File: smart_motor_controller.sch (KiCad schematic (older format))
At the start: 44 parts, among them J10 USB_B_Micro, J101 Conn_02x04_Odd_Even, J102 I2C_CONN, J103 CAN_CONN, J104 Conn_02x05_Odd_Even, J9 Input 12V, Q101 FDD6685, SW102 SW_NRST, SW103 SW_NRST, U2 STM32F405RGT6, U3 USBLC6-2SC6

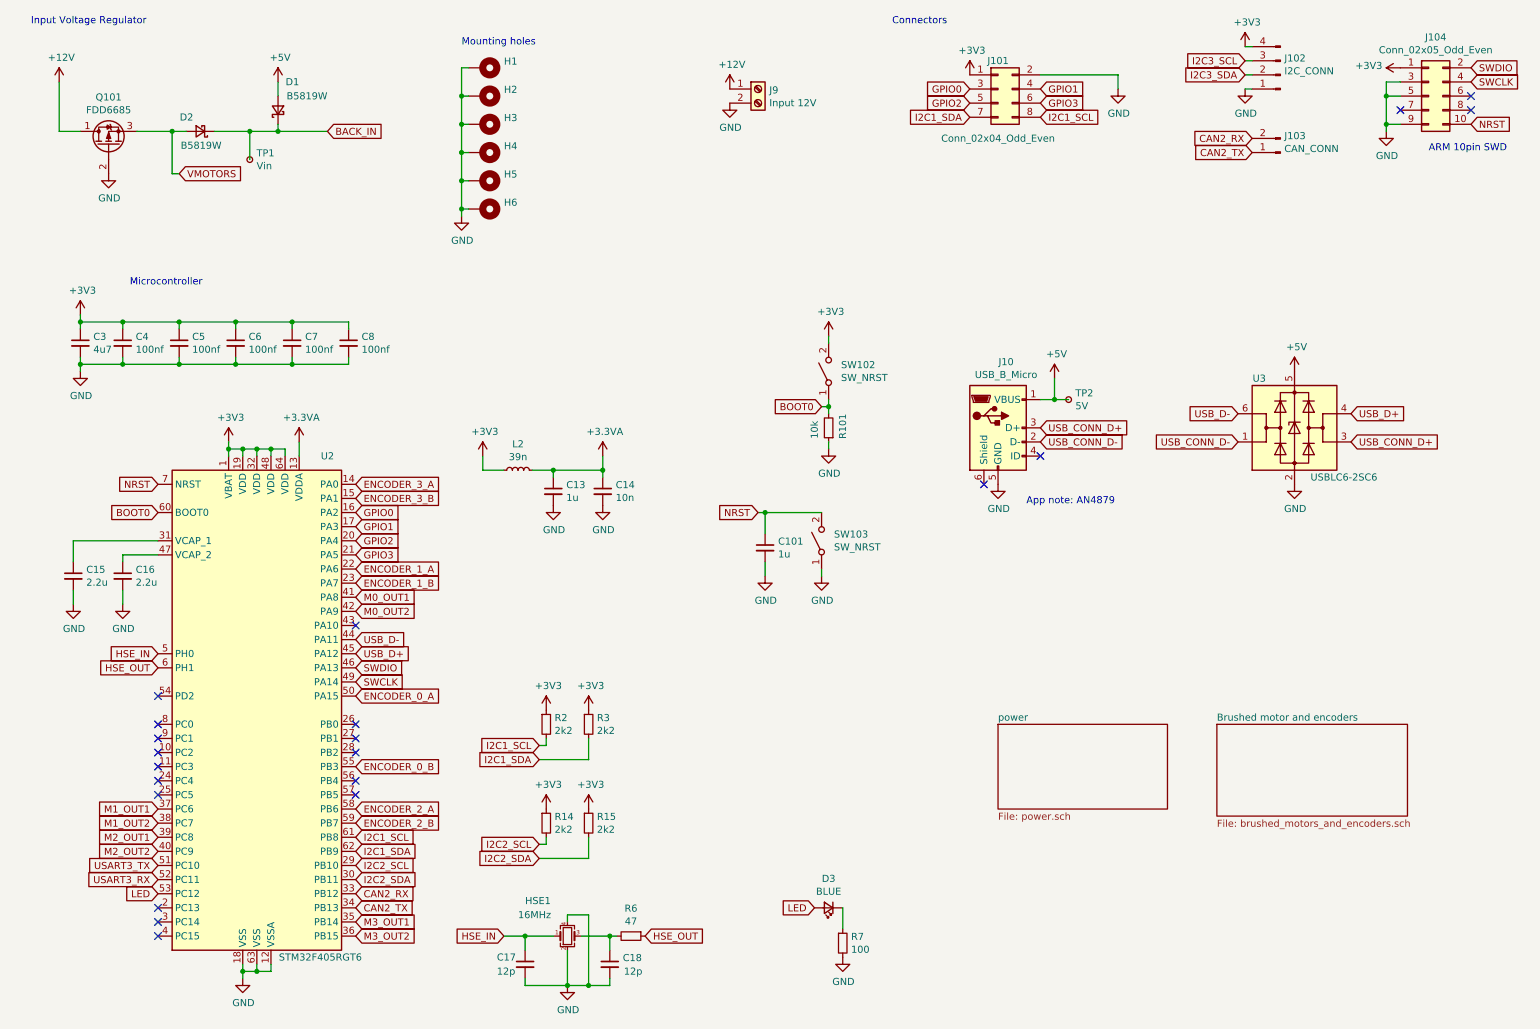
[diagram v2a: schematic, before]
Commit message: Layout
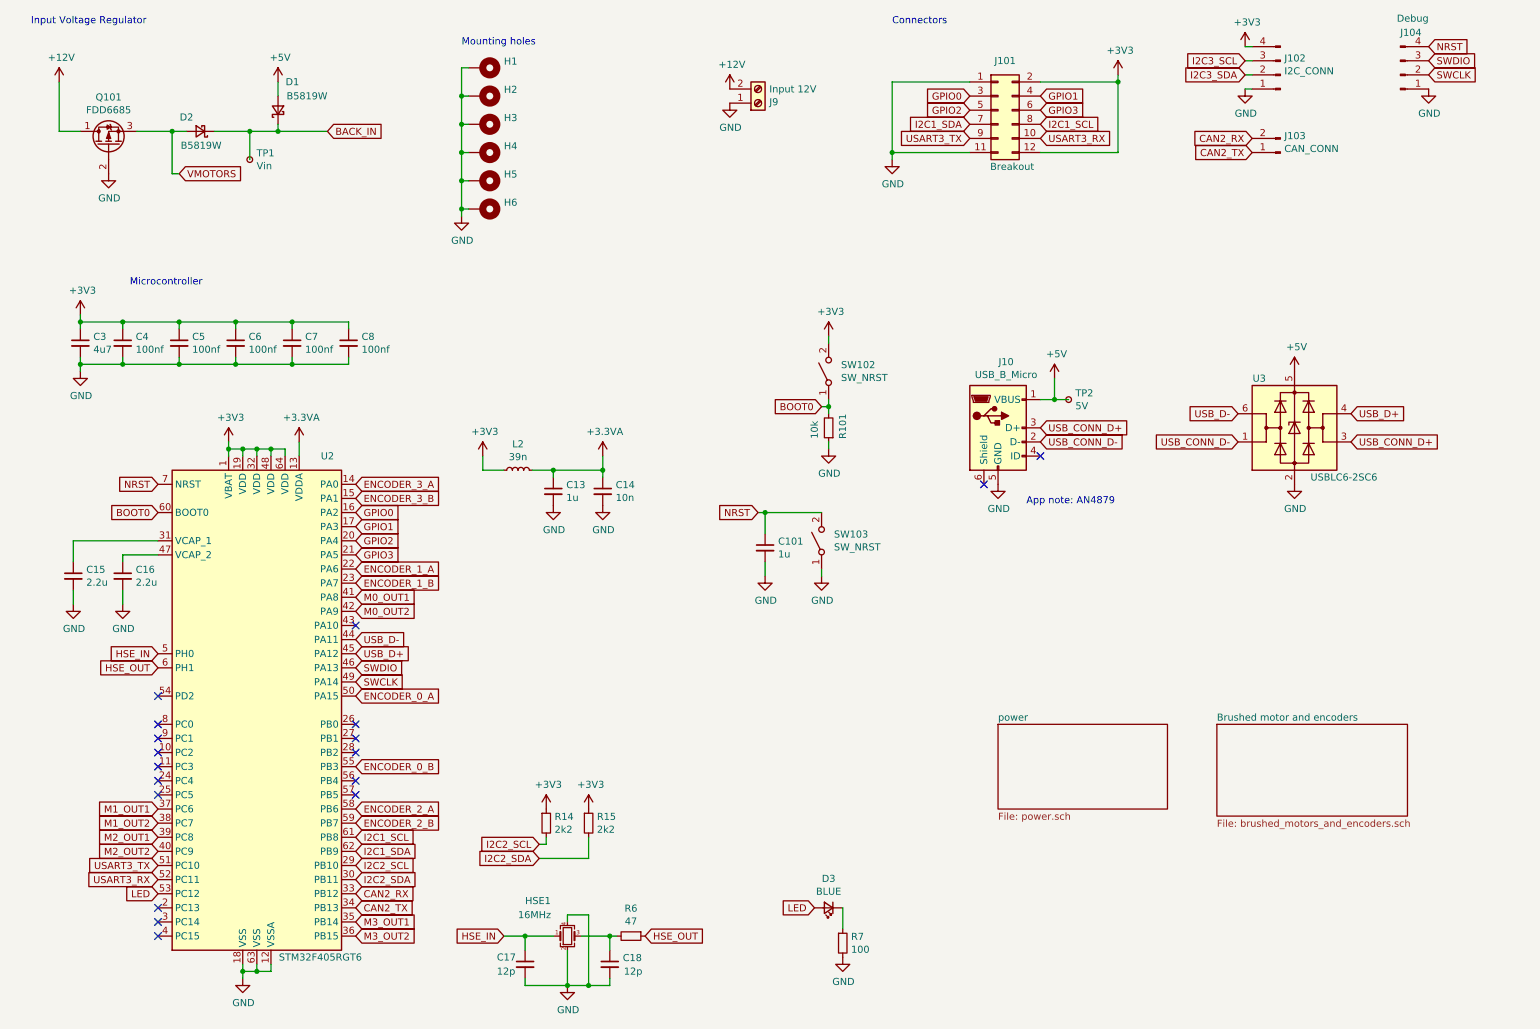
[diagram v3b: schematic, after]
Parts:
- removed J101: Conn_02x04_Odd_Even, Connector_PinHeader_2.54mm:PinHeader_2x04_P2.54mm_Vertical, symbol Connector_Generic:Conn_02x04_Odd_Even
- removed J104: Conn_02x05_Odd_Even, Connector_PinHeader_1.27mm:PinHeader_2x05_P1.27mm_Vertical_SMD, symbol Connector_Generic:Conn_02x05_Odd_Even
- removed R2, R3: 2k2, Resistor_THT:R_Axial_DIN0204_L3.6mm_D1.6mm_P5.08mm_Horizontal, symbol Device:R_Small
- added J101: Breakout, Connector_PinHeader_2.54mm:PinHeader_2x06_P2.54mm_Vertical, symbol Connector_Generic:Conn_02x06_Odd_Even
- added J104: Debug, Connector_PinHeader_2.54mm:PinHeader_1x04_P2.54mm_Vertical, symbol Connector:Conn_01x04_Male
- J9: footprint VsReality_Footprints:DB128L_5.08_2P_GN_S -> VsReality_Footprints:Ningbo_Kangnex_Elec_WJ128V_5_0_2P
- SW102, SW103: footprint (none) -> VsReality_Footprints:Diptronics MPTFP2-V-TR SMD 2.9x3.9x2mm; LCSC Part # (none) -> C495942
- TP1: footprint TestPoint:TestPoint_Pad_D2.0mm -> TestPoint:TestPoint_Pad_D1.5mm
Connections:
- net +12V: now also J9.2 (Pin_2); no longer J9.1 (Pin_1)
- net +3V3: now also J101.12 (Pin_12), J101.2 (Pin_2)
- net GND: now also J9.1 (Pin_1), J101.1 (Pin_1), J101.11 (Pin_11), J104.1 (Pin_1); no longer J9.2 (Pin_2)
- net GPIO0: now also J101.3 (Pin_3)
- net GPIO1: now also J101.4 (Pin_4)
- net GPIO2: now also J101.5 (Pin_5)
- net GPIO3: now also J101.6 (Pin_6)
- net I2C1_SCL: now also J101.8 (Pin_8)
- net I2C1_SDA: now also J101.7 (Pin_7)
- net NRST: now also J104.4 (Pin_4)
- net SWCLK: now also J104.2 (Pin_2)
- net SWDIO: now also J104.3 (Pin_3)
- net USART3_RX: now also J101.10 (Pin_10)
- net USART3_TX: now also J101.9 (Pin_9)
- no-connect marks 21 -> 18
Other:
- note removed: "ARM 10pin SWD\n"
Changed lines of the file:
@@
 Text GLabel 2900 5300 2    50   Input ~ 0
 SWCLK
-$Comp
-L Connector_Generic:Conn_02x05_Odd_Even J104
-U 1 1 6015F5C6
-P 10500 1150
-F 0 "J104" H 10550 1567 50  0000 C CNN
-F 1 "Conn_02x05_Odd_Even" H 10550 1476 50  0000 C CNN
-F 2 "Connector_PinHeader_1.27mm:PinHeader_2x05_P1.27mm_Vertical_SMD" H 10500 1150 50  0001 C CNN
-F 3 "~" H 10500 1150 50  0001 C CNN
-	1    10500 1150
-	1    0    0    -1
-$EndComp
-$Comp
-L power:GND #PWR07
-U 1 1 60160243
-P 10200 1400
-F 0 "#PWR07" H 10200 1150 50  0001 C CNN
-F 1 "GND" H 10205 1227 50  0000 C CNN
-F 2 "" H 10200 1400 50  0001 C CNN
-F 3 "" H 10200 1400 50  0001 C CNN
-	1    10200 1400
-	1    0    0    -1
-$EndComp
-Wire Wire Line
-	10300 1050 10200 1050
-Wire Wire Line
-	10200 1050 10200 1150
-Wire Wire Line
-	10300 1150 10200 1150
-Connection ~ 10200 1150
-Wire Wire Line
-	10200 1150 10200 1350
-Wire Wire Line
-	10300 1350 10200 1350
-Connection ~ 10200 1350
-Wire Wire Line
-	10200 1350 10200 1400
-$Comp
-L power:+3V3 #PWR05
-U 1 1 6016A0E3
-P 10300 950
-F 0 "#PWR05" H 10300 800 50  0001 C CNN
-F 1 "+3V3" V 10315 1078 50  0000 L CNN
-F 2 "" H 10300 950 50  0001 C CNN
-F 3 "" H 10300 950 50  0001 C CNN
-	1    10300 950
-	0    -1   -1   0
-$EndComp
-NoConn ~ 10300 1250
-NoConn ~ 10800 1250
-Text GLabel 10800 1350 2    50   Input ~ 0
-NRST
-Text GLabel 10800 1050 2    50   Input ~ 0
-SWCLK
-Text GLabel 10800 950  2    50   Input ~ 0
-SWDIO
-Text Notes 10500 1550 0    50   ~ 0
-ARM 10pin SWD\n
 Text GLabel 2900 6500 2    50   Input ~ 0
 I2C1_SDA
@@
 Text Notes 1300 2500 0    50   ~ 0
 Microcontroller
-Text GLabel 7750 1300 2    50   Input ~ 0
+Text GLabel 7750 1350 2    50   Input ~ 0
 I2C1_SCL
-Text GLabel 7250 1300 0    50   Input ~ 0
+Text GLabel 7250 1350 0    50   Input ~ 0
 I2C1_SDA
 $Comp
 L power:+3V3 #PWR06
 U 1 1 6026AA86
-P 7250 1000
-F 0 "#PWR06" H 7250 850 50  0001 C CNN
-F 1 "+3V3" H 7265 1173 50  0000 C CNN
-F 2 "" H 7250 1000 50  0001 C CNN
-F 3 "" H 7250 1000 50  0001 C CNN
-	1    7250 1000
-	1    0    0    -1
-$EndComp
-$Comp
-L power:GND #PWR09
-U 1 1 6026AECF
-P 8300 1100
-F 0 "#PWR09" H 8300 850 50  0001 C CNN
-F 1 "GND" H 8305 927 50  0000 C CNN
-F 2 "" H 8300 1100 50  0001 C CNN
-F 3 "" H 8300 1100 50  0001 C CNN
-	1    8300 1100
+P 8300 1000
+F 0 "#PWR06" H 8300 850 50  0001 C CNN
+F 1 "+3V3" H 8315 1173 50  0000 C CNN
+F 2 "" H 8300 1000 50  0001 C CNN
+F 3 "" H 8300 1000 50  0001 C CNN
+	1    8300 1000
 	1    0    0    -1
 $EndComp
@@
 Text GLabel 2900 6900 2    50   Input ~ 0
 CAN2_TX
-NoConn ~ 10800 1150
 $Comp
 L Connector:Screw_Terminal_01x02 J9
 U 1 1 60318CBC
-P 5750 1100
-F 0 "J9" H 5830 1092 50  0000 L CNN
-F 1 "Input 12V" H 5830 1001 50  0000 L CNN
-F 2 "VsReality_Footprints:DB128L_5.08_2P_GN_S" H 5750 1100 50  0001 C CNN
-F 3 "~" H 5750 1100 50  0001 C CNN
-	1    5750 1100
-	1    0    0    -1
+P 5750 1200
+F 0 "J9" H 5830 1192 50  0000 L CNN
+F 1 "Input 12V" H 5830 1101 50  0000 L CNN
+F 2 "VsReality_Footprints:Ningbo_Kangnex_Elec_WJ128V_5_0_2P" H 5750 1200 50  0001 C CNN
+F 3 "~" H 5750 1200 50  0001 C CNN
+	1    5750 1200
+	1    0    0    1
 $EndComp
 $Comp
@@
 	1    0    0    -1
 $EndComp
-Wire Wire Line
-	4550 5850 4550 5700
-Wire Wire Line
-	4200 5850 4550 5850
-Wire Wire Line
-	4250 5750 4200 5750
-Wire Wire Line
-	4250 5700 4250 5750
-Text GLabel 4200 5750 0    50   Input ~ 0
-I2C1_SCL
-Text GLabel 4200 5850 0    50   Input ~ 0
-I2C1_SDA
-$Comp
-L Device:R_Small R2
-U 1 1 60262C5F
-P 4250 5600
-F 0 "R2" H 4309 5646 50  0000 L CNN
-F 1 "2k2" H 4309 5555 50  0000 L CNN
-F 2 "Resistor_THT:R_Axial_DIN0204_L3.6mm_D1.6mm_P5.08mm_Horizontal" H 4250 5600 50  0001 C CNN
-F 3 "~" H 4250 5600 50  0001 C CNN
-F 4 "" H 4250 5600 50  0001 C CNN "LCSC Part #"
-	1    4250 5600
-	1    0    0    -1
-$EndComp
-$Comp
-L power:+3V3 #PWR020
-U 1 1 60264184
-P 4550 5500
-F 0 "#PWR020" H 4550 5350 50  0001 C CNN
-F 1 "+3V3" H 4565 5673 50  0000 C CNN
-F 2 "" H 4550 5500 50  0001 C CNN
-F 3 "" H 4550 5500 50  0001 C CNN
-	1    4550 5500
-	1    0    0    -1
-$EndComp
-$Comp
-L power:+3V3 #PWR019
-U 1 1 602635FF
-P 4250 5500
-F 0 "#PWR019" H 4250 5350 50  0001 C CNN
-F 1 "+3V3" H 4265 5673 50  0000 C CNN
-F 2 "" H 4250 5500 50  0001 C CNN
-F 3 "" H 4250 5500 50  0001 C CNN
-	1    4250 5500
-	1    0    0    -1
-$EndComp
-$Comp
-L Device:R_Small R3
-U 1 1 6026341E
-P 4550 5600
-F 0 "R3" H 4609 5646 50  0000 L CNN
-F 1 "2k2" H 4609 5555 50  0000 L CNN
-F 2 "Resistor_THT:R_Axial_DIN0204_L3.6mm_D1.6mm_P5.08mm_Horizontal" H 4550 5600 50  0001 C CNN
-F 3 "~" H 4550 5600 50  0001 C CNN
-F 4 "" H 4550 5600 50  0001 C CNN "LCSC Part #"
-	1    4550 5600
-	1    0    0    -1
-$EndComp
 Text GLabel 2700 1400 2    50   Input ~ 0
 BACK_IN
@@
 Text GLabel 2900 4400 2    50   Input ~ 0
 GPIO3
-Text GLabel 7250 1100 0    50   Input ~ 0
+Text GLabel 7250 1150 0    50   Input ~ 0
 GPIO0
-Text GLabel 7750 1100 2    50   Input ~ 0
+Text GLabel 7750 1150 2    50   Input ~ 0
 GPIO1
-Text GLabel 7750 1200 2    50   Input ~ 0
+Text GLabel 7750 1250 2    50   Input ~ 0
 GPIO3
 Wire Wire Line
@@
 F 0 "TP1" H 2198 1646 50  0000 L CNN
 F 1 "Vin" H 2198 1555 50  0000 L CNN
-F 2 "TestPoint:TestPoint_Pad_D2.0mm" H 2350 1600 50  0001 C CNN
+F 2 "TestPoint:TestPoint_Pad_D1.5mm" H 2350 1600 50  0001 C CNN
 F 3 "~" H 2350 1600 50  0001 C CNN
 	1    2150 1600
@@
 NoConn ~ 2900 6000
 NoConn ~ 2900 6100
-$Comp
-L Connector_Generic:Conn_02x04_Odd_Even J101
-U 1 1 60A454AD
-P 7450 1100
-F 0 "J101" H 7450 1300 50  0000 C CNN
-F 1 "Conn_02x04_Odd_Even" H 7450 750 50  0000 C CNN
-F 2 "Connector_PinHeader_2.54mm:PinHeader_2x04_P2.54mm_Vertical" H 7450 1100 50  0001 C CNN
-F 3 "~" H 7450 1100 50  0001 C CNN
-	1    7450 1100
-	1    0    0    -1
-$EndComp
-Text GLabel 7250 1200 0    50   Input ~ 0
+Text GLabel 7250 1250 0    50   Input ~ 0
 GPIO2
 Wire Wire Line
-	8300 1000 8300 1100
-Wire Wire Line
-	7750 1000 8300 1000
+	7750 1050 8300 1050
 Wire Wire Line
 	800  1050 800  1400
@@
 F 0 "SW103" V 6246 4212 50  0000 R CNN
 F 1 "SW_NRST" V 6155 4212 50  0000 R CNN
-F 2 "" H 6200 4300 50  0001 C CNN
+F 2 "VsReality_Footprints:Diptronics MPTFP2-V-TR SMD 2.9x3.9x2mm" H 6200 4300 50  0001 C CNN
 F 3 "~" H 6200 4300 50  0001 C CNN
+F 4 "C495942" H 6200 4300 50  0001 C CNN "LCSC Part #"
 	1    6200 4300
 	0    -1   -1   0
@@
 F 0 "SW102" V 6296 3012 50  0000 R CNN
 F 1 "SW_NRST" V 6205 3012 50  0000 R CNN
-F 2 "" H 6250 3100 50  0001 C CNN
+F 2 "VsReality_Footprints:Diptronics MPTFP2-V-TR SMD 2.9x3.9x2mm" H 6250 3100 50  0001 C CNN
 F 3 "~" H 6250 3100 50  0001 C CNN
+F 4 "C495942" H 6250 3100 50  0001 C CNN "LCSC Part #"
 	1    6250 3100
 	0    -1   -1   0
@@
 	-1   0    0    1
 $EndComp
+$Comp
+L Connector_Generic:Conn_02x06_Odd_Even J101
+U 1 1 60C56406
+P 7450 1250
+F 0 "J101" H 7500 1600 50  0000 C CNN
+F 1 "Breakout" H 7550 850 50  0000 C CNN
+F 2 "Connector_PinHeader_2.54mm:PinHeader_2x06_P2.54mm_Vertical" H 7450 1250 50  0001 C CNN
+F 3 "~" H 7450 1250 50  0001 C CNN
+	1    7450 1250
+	1    0    0    -1
+$EndComp
+$Comp
+L power:GND #PWR0121
+U 1 1 60C59A47
+P 6700 1600
+F 0 "#PWR0121" H 6700 1350 50  0001 C CNN
+F 1 "GND" H 6705 1427 50  0000 C CNN
+F 2 "" H 6700 1600 50  0001 C CNN
+F 3 "" H 6700 1600 50  0001 C CNN
+	1    6700 1600
+	1    0    0    -1
+$EndComp
+Wire Wire Line
+	7750 1550 8300 1550
+Wire Wire Line
+	7250 1550 6700 1550
+Text GLabel 7250 1450 0    50   Input ~ 0
+USART3_TX
+Text GLabel 7750 1450 2    50   Input ~ 0
+USART3_RX
+Wire Wire Line
+	8300 1050 8300 1550
+Wire Wire Line
+	7250 1050 6700 1050
+Wire Wire Line
+	6700 1050 6700 1550
+Wire Wire Line
+	8300 1050 8300 1000
+Connection ~ 8300 1050
+Wire Wire Line
+	6700 1600 6700 1550
+Connection ~ 6700 1550
+$Comp
+L Connector:Conn_01x04_Male J104
+U 1 1 60C6E515
+P 10300 1000
+F 0 "J104" H 10450 700 50  0000 R CNN
+F 1 "Debug" H 10500 600 50  0000 R CNN
+F 2 "Connector_PinHeader_2.54mm:PinHeader_1x04_P2.54mm_Vertical" H 10300 1000 50  0001 C CNN
+F 3 "~" H 10300 1000 50  0001 C CNN
+	1    10300 1000
+	1    0    0    1
+$EndComp
+$Comp
+L power:GND #PWR0122
+U 1 1 60C6EF67
+P 10500 1100
+F 0 "#PWR0122" H 10500 850 50  0001 C CNN
+F 1 "GND" H 10505 927 50  0000 C CNN
+F 2 "" H 10500 1100 50  0001 C CNN
+F 3 "" H 10500 1100 50  0001 C CNN
+	1    10500 1100
+	1    0    0    -1
+$EndComp
+Text GLabel 10500 800  2    50   Input ~ 0
+NRST
+Text GLabel 10500 1000 2    50   Input ~ 0
+SWCLK
+Text GLabel 10500 900  2    50   Input ~ 0
+SWDIO
 $EndSCHEMATC
